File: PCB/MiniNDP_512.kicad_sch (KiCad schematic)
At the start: 20 parts, among them J1 Conn_02x20_Odd_Even, U1 HC161, U2 HC161, U3 HC161, U4 HC138, U5 HC374, U6 AS6C4008, U7 1G32, U8 1G79

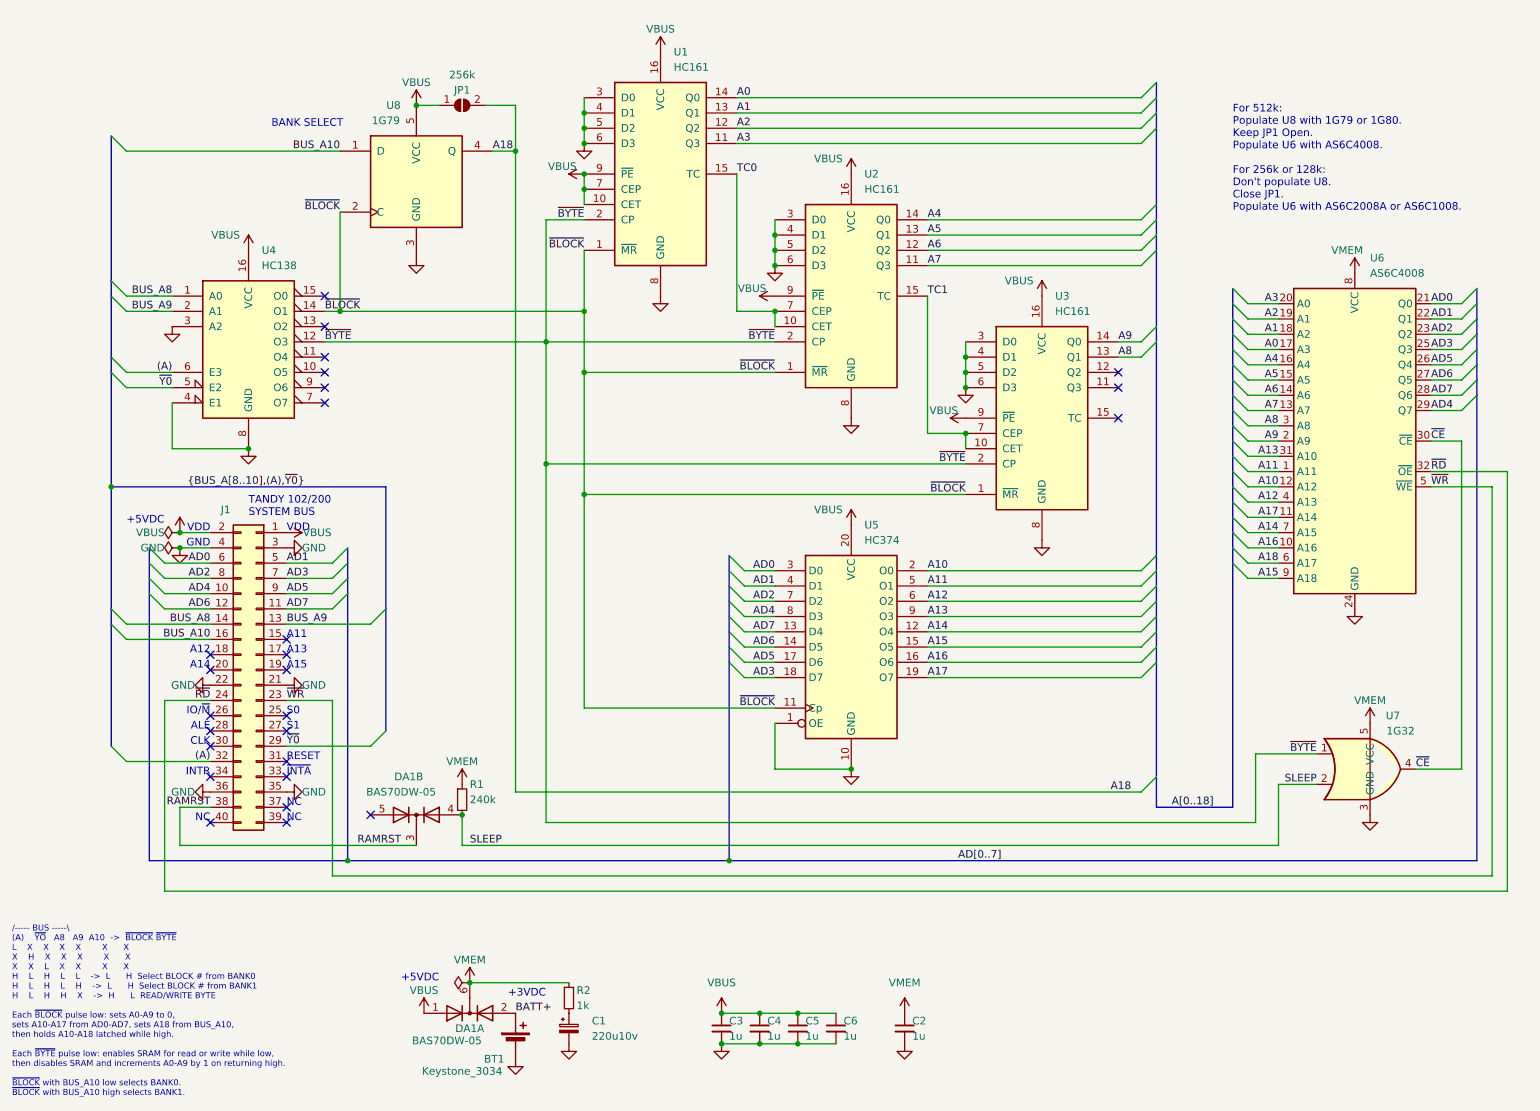
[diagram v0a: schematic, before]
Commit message: 1M_B & 512_B
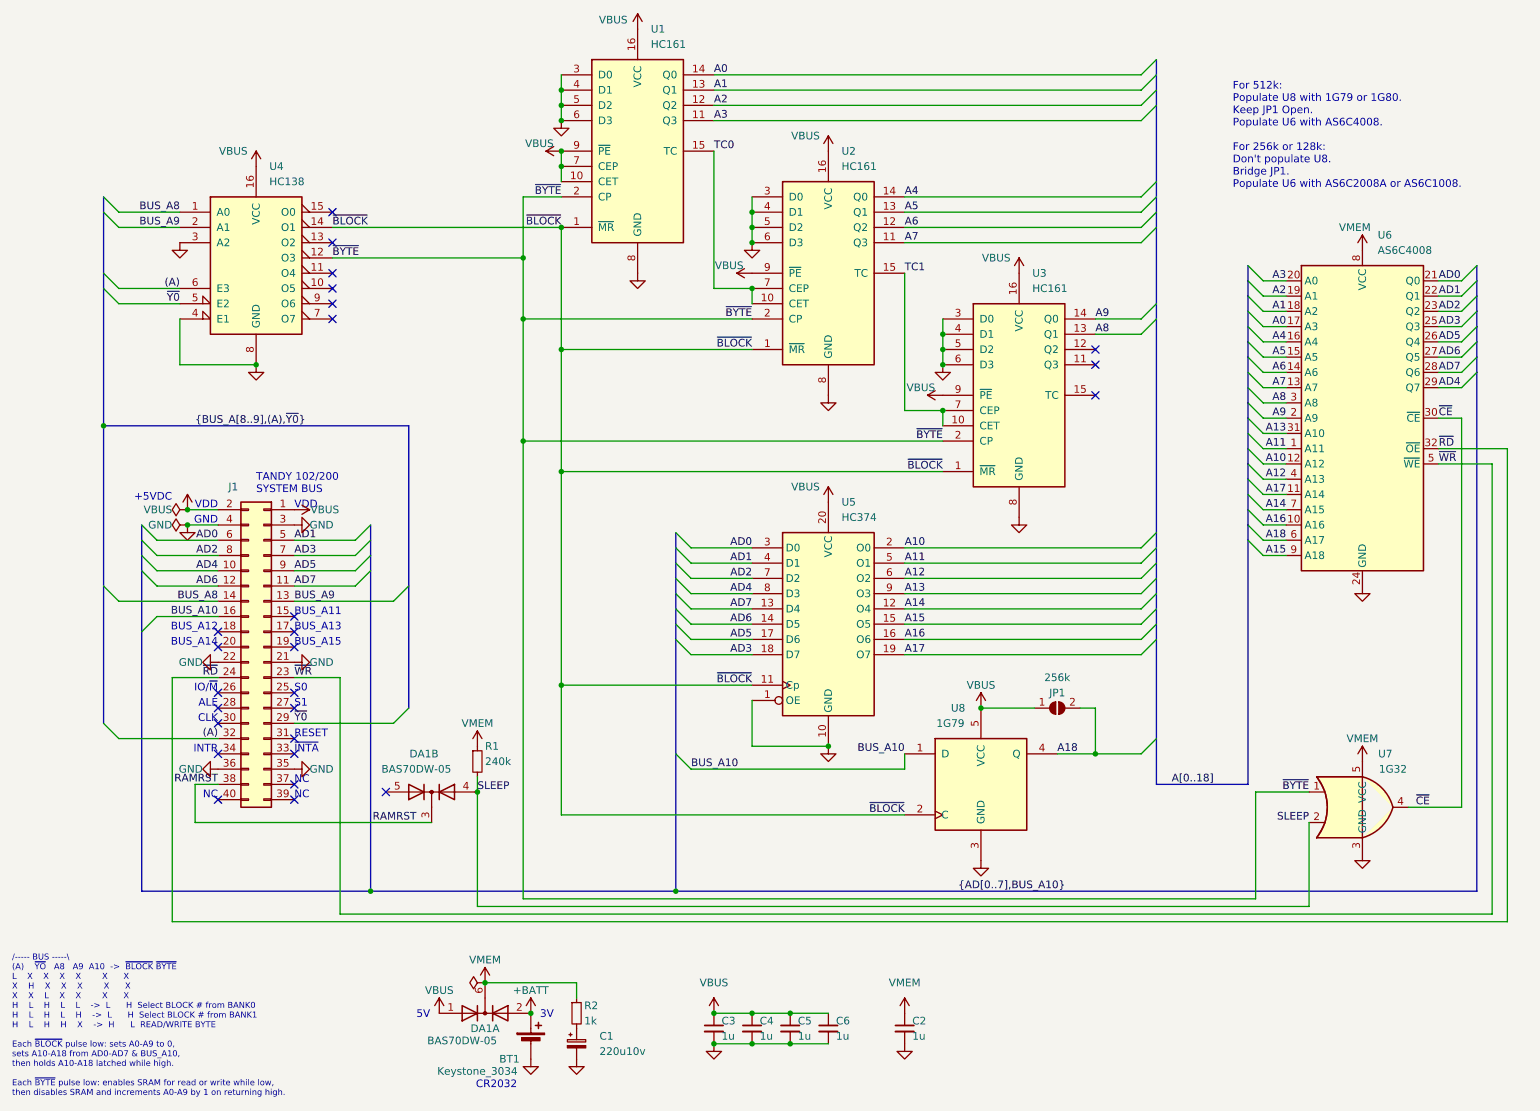
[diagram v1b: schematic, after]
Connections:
- net BATT+ renamed +BATT
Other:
- note added: "/----- BUS -----\ (A) ~{YO} A8 A9 A10 -> ~{BLOCK} ~{BYTE} L X X X X X X X H X X X X X X X L X X X X H L H L L -> L H Select BLOCK # from BANK0 H L H L H -> L H Select BLOCK # from BANK1 H L H H X -> H L READ/WRITE BYTE Each ~{BLOCK} pulse low: sets A0-A9 to 0, sets A10-A18 from AD0-AD7 & BUS_A10, then holds A10-A18 latched while high. Each ~{BYTE} pulse low: enables SRAM for read or write while l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"
- note added: "3V"
- note added: "5V"
- note added: "BUS_A11"
- note added: "BUS_A12"
- note added: "BUS_A13"
- note added: "BUS_A14"
- note added: "BUS_A15"
- note added: "CR2032"
- note added: "For 512k: Populate U8 with 1G79 or 1G80. Keep JP1 Open. Populate U6 with AS6C4008. For 256k or 128k: Don't populate U8. Bridge JP1. Populate U6 with AS6C2008A or AS6C1008."
- note removed: "+3VDC"
- note removed: "/----- BUS -----\ (A) ~{YO} A8 A9 A10 -> ~{BLOCK} ~{BYTE} L X X X X X X X H X X X X X X X L X X X X H L H L L -> L H Select BLOCK # from BANK0 H L H L H -> L H Select BLOCK # from BANK1 H L H H X -> H L READ/WRITE BYTE Each ~{BLOCK} pulse low: sets A0-A9 to 0, sets A10-A17 from AD0-AD7, sets A18 from BUS_A10, then holds A10-A18 latched while high. Each ~{BYTE} pulse low: enables SRAM for read or 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"
- note removed: "A11"
- note removed: "A12"
- note removed: "A13"
- note removed: "A14"
- note removed: "A15"
- note removed: "BANK SELECT"
- note removed: "For 512k: Populate U8 with 1G79 or 1G80. Keep JP1 Open. Populate U6 with AS6C4008. For 256k or 128k: Don't populate U8. Close JP1. Populate U6 with AS6C2008A or AS6C1008."
- moved on the sheet: BT1, C1, C3, C4, C5, C6, DA1A, DA1B, J1, R1, R2, U1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
